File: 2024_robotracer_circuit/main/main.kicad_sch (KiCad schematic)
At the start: 18 parts, among them J1 Conn_01x06, J2 Conn_02x05_Odd_Even, J3 Conn_02x05_Odd_Even, SW1 SW_Push, U1 STM32F405RGTx

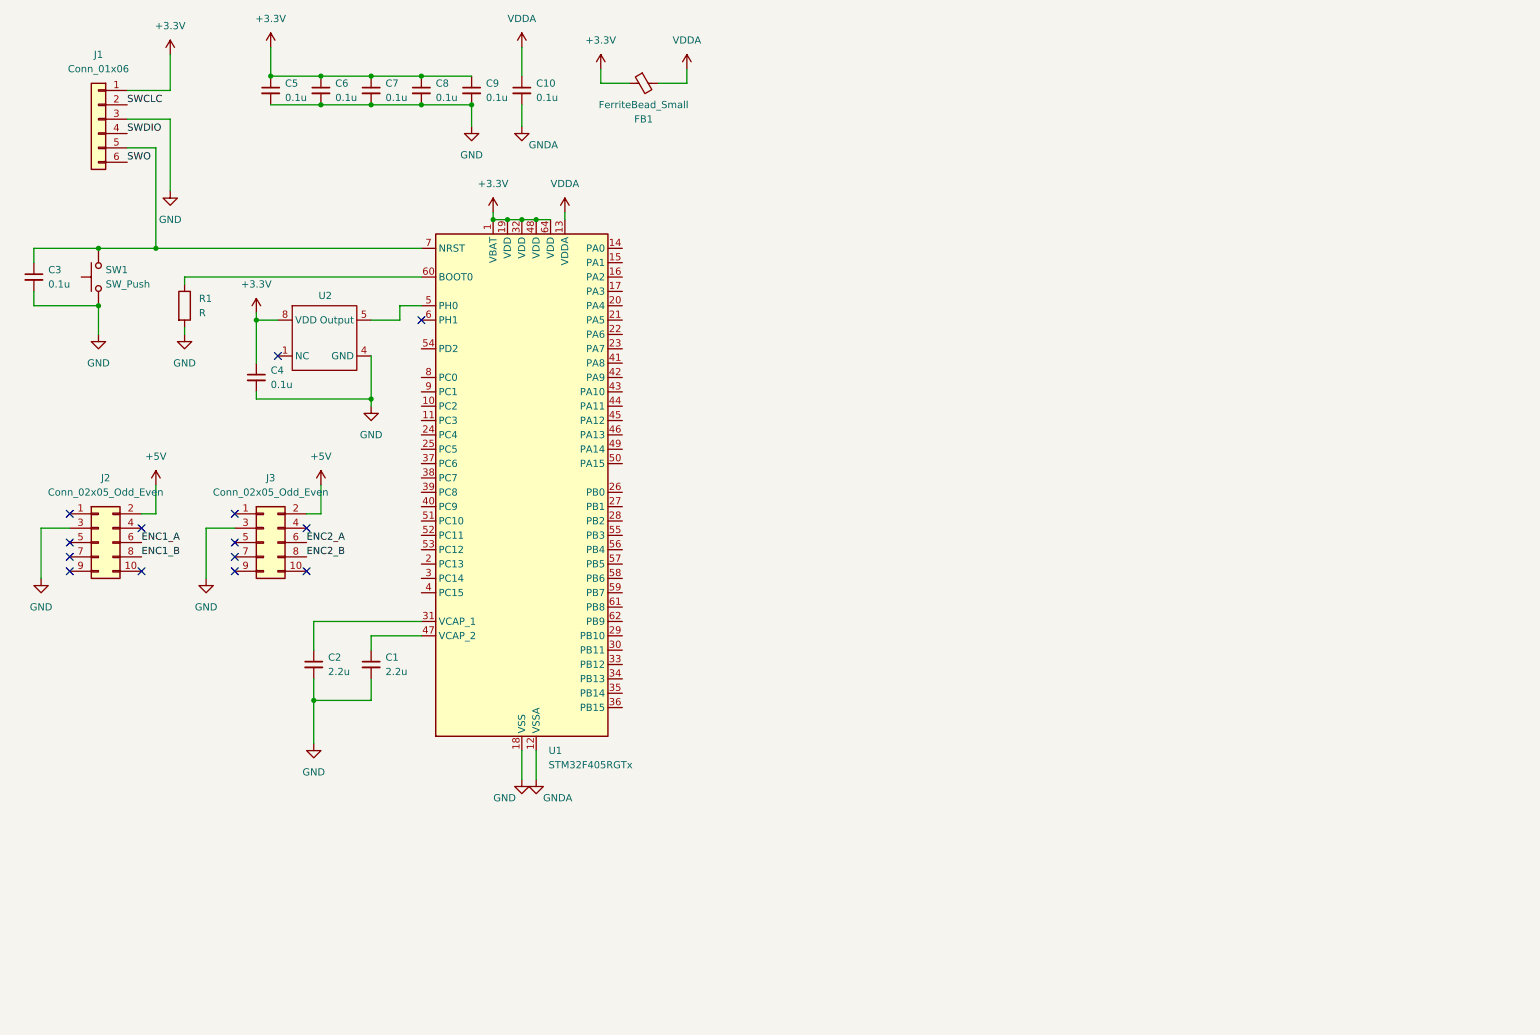
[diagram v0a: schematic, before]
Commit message: 進めた
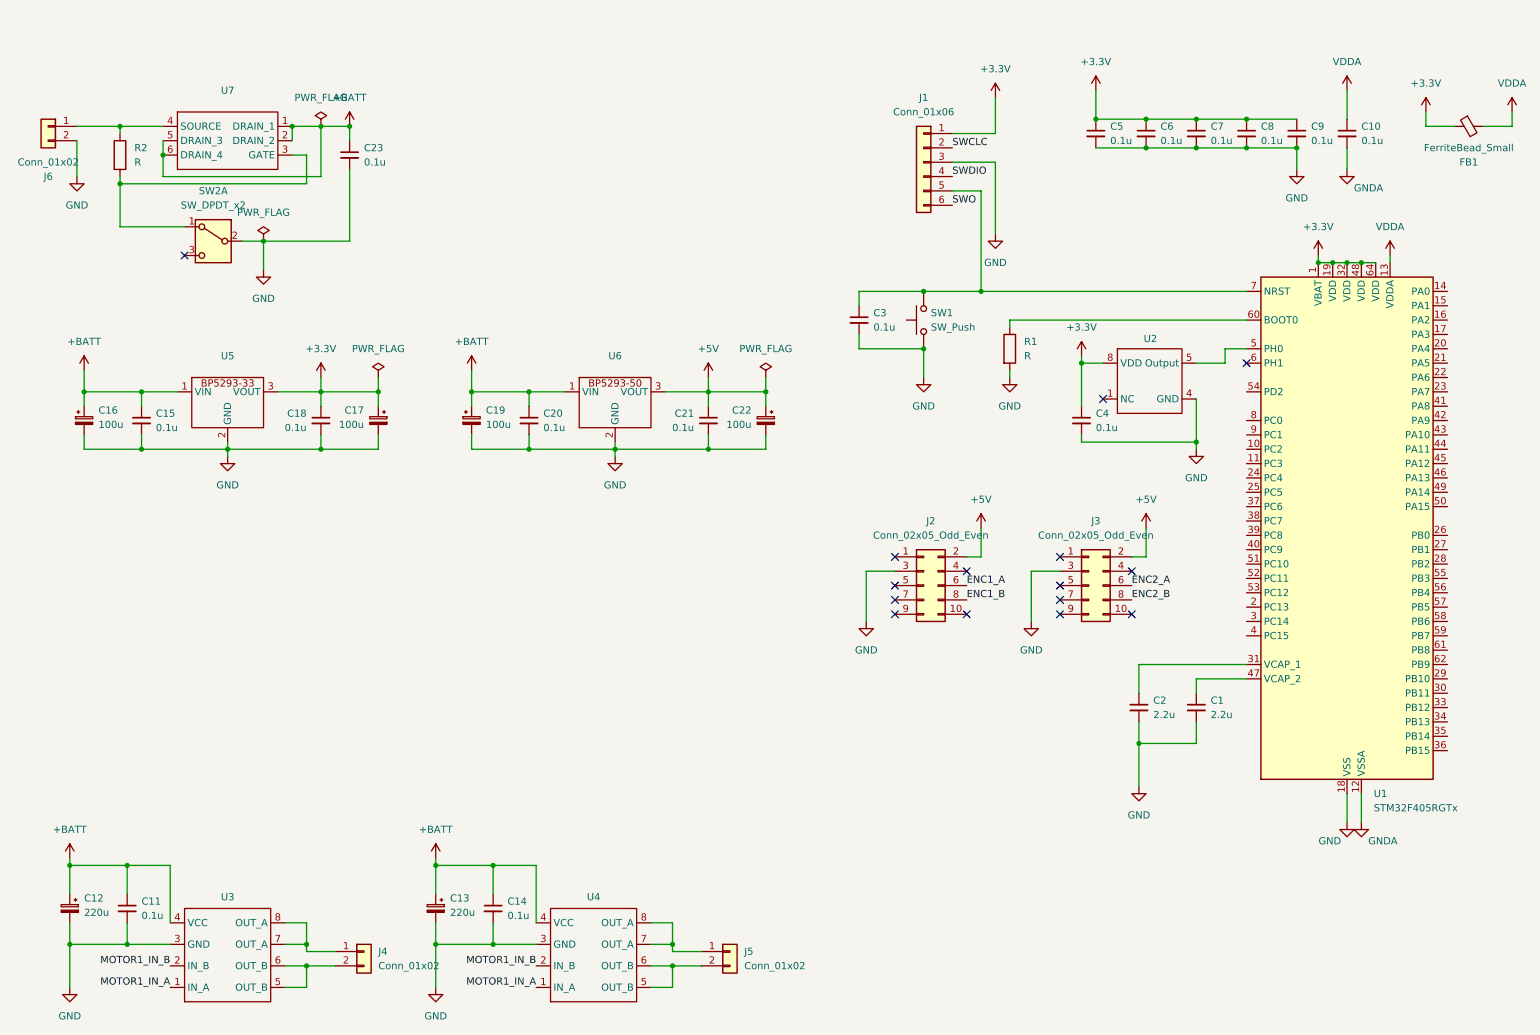
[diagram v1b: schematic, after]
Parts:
- added C11, C14, C15, C18, C20, C21, C23: 0.1u, symbol Device:C_Small
- added C12, C13: 220u, symbol Device:C_Polarized_Small
- added C16, C17, C19, C22: 100u, symbol Device:C_Polarized_Small
- added J4, J5, J6: Conn_01x02, symbol Connector_Generic:Conn_01x02
- added R2: R, symbol Device:R
- added SW2: SW_DPDT_x2, symbol Switch:SW_DPDT_x2
- added U3, U4: ~, symbol mylib:AM2837
- added U5: ~, symbol mylib:BP5293-33
- added U6: ~, symbol mylib:BP5293-50
- added U7: ~, symbol mylib:SSM6J808R
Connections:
- net +3.3V: now also C17.1, C18.1, U5.3 (VOUT)
- net +5V: now also C21.1, C22.1, U6.3 (VOUT)
- net GND: now also C11.2, C12.2, C13.2, C14.2, C15.2, C16.2, C17.2, C18.2, C19.2, C20.2, C21.2, C22.2, C23.2, J6.2 (Pin_2), SW2.2 (B), U3.3 (GND), U4.3 (GND), U5.2 (GND), U6.2 (GND)
- new net: J6.1 (Pin_1), R2.1, U7.4 (SOURCE)
- new net: J4.1 (Pin_1), U3.7 (OUT_A), U3.8 (OUT_A)
- new net: J4.2 (Pin_2), U3.5 (OUT_B), U3.6 (OUT_B)
- new net: R2.2, SW2.1 (A), U7.3 (GATE)
- new net: J5.2 (Pin_2), U4.5 (OUT_B), U4.6 (OUT_B)
- new net: J5.1 (Pin_1), U4.7 (OUT_A), U4.8 (OUT_A)
- new net +BATT: C11.1, C12.1, C13.1, C14.1, C15.1, C16.1, C19.1, C20.1, C23.1, U3.4 (VCC), U4.4 (VCC), U5.1 (VIN), U6.1 (VIN), U7.1 (DRAIN_1), U7.2 (DRAIN_2), U7.5 (DRAIN_3), U7.6 (DRAIN_4)
- new net MOTOR1_IN_A: U3.1 (IN_A), U4.1 (IN_A)
- new net MOTOR1_IN_B: U3.2 (IN_B), U4.2 (IN_B)
- no-connect marks 14 -> 15
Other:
- moved on the sheet: C1, C10, C2, C3, C4, C5, C6, C7, C8, C9, FB1, J1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

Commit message: 途中
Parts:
- added BZ1: Buzzer, symbol Device:Buzzer
- added C24: 220u, symbol Device:C_Polarized_Small
- added C25: 0.1u, symbol Device:C_Small
- added C26, C27: 100u, symbol Device:C_Polarized_Small
- added D1: D, symbol Device:D
- added D2, D3, D4: LED_Small, symbol Device:LED_Small
- added J10, J11: Conn_01x03, symbol Connector_Generic:Conn_01x03
- added J7: Micro_SD_Card_Det1, symbol Connector:Micro_SD_Card_Det1
- added J8: Conn_01x04, symbol Connector_Generic:Conn_01x04
- added J9: Conn_01x06, symbol Connector_Generic:Conn_01x06
- added R11, R12, R13, R14, R15, R16, R17: 22k, symbol Device:R_Small
- added R18, R19, R20, R21, R22, R25, R28: 47k, symbol Device:R_Small
- added R23, R24, R31, R32, R33: R_Small, symbol Device:R_Small
- added R26, R29, R3, R5, R7, R9: 4.7, symbol Device:R_Small
- added R34, R35, R36, R37, R38, R39, R4, R6: 1k, symbol Device:R_Small
- added U10, U12, U14, U17, U18, U20, U9: ~, symbol mylib:MTN2306AN3
- added U11, U13, U15, U19, U21, U8: ~, symbol mylib:LBR-127HLD
- added U16: ~, symbol mylib:AE-BMX055
- J4, J5: value Conn_01x02 -> PA_2p
- J6: value Conn_01x02 -> XT_2p
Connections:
- net +3.3V: now also C24.1, C25.1, J7.4 (VDD), J8.1 (Pin_1), R11.1, R12.1, R13.1, R14.1, R15.1, R16.1, R32.1, R34.1, R35.1, U16.4 (3V3)
- net +5V: now also J10.1 (Pin_1), J11.1 (Pin_1), J9.1 (Pin_1), R33.1, R36.1, R37.1, R38.1, R39.1, R4.1, R6.1, U11.1 (anode), U13.1 (anode), U15.1 (anode), U19.1 (anode), U21.1 (anode), U8.1 (anode)
- net +BATT: now also BZ1.1 (+), C26.1, C27.1, D1.1 (K), R23.1, R31.1
- net GND: now also C24.2, C25.2, C26.2, C27.2, D2.1 (K), D3.1 (K), D4.1 (K), J10.3 (Pin_3), J11.3 (Pin_3), J7.10 (SHIELD), J7.6 (VSS), J8.4 (Pin_4), J9.6 (Pin_6), R17.2, R18.2, R19.2, R20.2, R21.2, R22.2, R24.2, R25.2, R28.2, U10.3 (S), U11.3 (E), U12.3 (S), U13.3 (E), U14.3 (S), U15.3 (E), U16.1 (GND), U17.3 (S), U18.3 (S), U19.3 (E), U20.3 (S), U21.3 (E), U8.3 (E), U9.3 (S)
- new net: R29.1, U21.2 (cathode)
- new net: R29.2, U20.2 (D)
- new net: R26.1, U19.2 (cathode)
- new net: R26.2, U18.2 (D)
- new net: R3.2, U9.2 (D)
- new net: R5.1, U11.2 (cathode)
- new net: D3.2 (A), R32.2
- new net: R3.1, U8.2 (cathode)
- new net: J7.1 (DAT2), R16.2
- new net: R9.1, U15.2 (cathode)
- new net: R9.2, U14.2 (D)
- new net: D4.2 (A), R33.2
- new net: R5.2, U10.2 (D)
- new net: J7.8 (DAT1), R12.2
- new net: D2.2 (A), R31.2
- new net: BZ1.2 (-), D1.2 (A), U17.2 (D)
- new net: J7.2 (DAT3/CD), R15.2
- new net: R7.1, U13.2 (cathode)
- new net: R7.2, U12.2 (D)
- new net BATT_REF: R23.2, R24.1
- new net BZ_PWM: R22.1, U17.1 (G)
- new net IMU_SCL: U16.3 (SCL)
- new net IMU_SDA: U16.2 (SDA)
- new net LCD_SCL: J8.3 (Pin_3), R35.2
- new net LCD_SDA: J8.2 (Pin_2), R34.2
- new net SDIO_CK: J7.5 (CLK), R17.1
- new net SDIO_CMD: J7.3 (CMD), R14.2
- new net SDIO_D0: J7.7 (DAT0), R13.2
- new net SDIO_SW: J7.9 (DET), R11.2
- new net SENSOR0_ADC: J9.2 (Pin_2), R36.2, U8.4 (C)
- new net SENSOR0_PWM: R18.1, U9.1 (G)
- new net SENSOR1_ADC: J9.3 (Pin_3), R37.2, U11.4 (C)
- new net SENSOR1_PWM: R19.1, U10.1 (G)
- new net SENSOR2_ADC: J9.4 (Pin_4), R38.2, U13.4 (C)
- new net SENSOR2_PWM: R20.1, U12.1 (G)
- new net SENSOR3_ADC: J9.5 (Pin_5), R39.2, U15.4 (C)
- new net SENSOR3_PWM: R21.1, U14.1 (G)
- new net SENSOR_L_ADC: J10.2 (Pin_2), R4.2, U19.4 (C)
- new net SENSOR_L_PWM: R25.1, U18.1 (G)
- new net SENSOR_R_ADC: J11.2 (Pin_2), R6.2, U21.4 (C)
- new net SENSOR_R_PWM: R28.1, U20.1 (G)
- no-connect marks 15 -> 17
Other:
- moved on the sheet: C1, C10, C11, C12, C13, C14, C15, C16, C17, C18, C19, C2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
